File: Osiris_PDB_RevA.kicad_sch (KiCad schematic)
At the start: 22 parts, among them J1 XT60, Q1 ISC015N06NM5LF2, Q2 ISC015N06NM5LF2, U1 LTC4368IMS-1-PBF, U2 INA228AIDGSR, U3 TPS7A1633DGNR

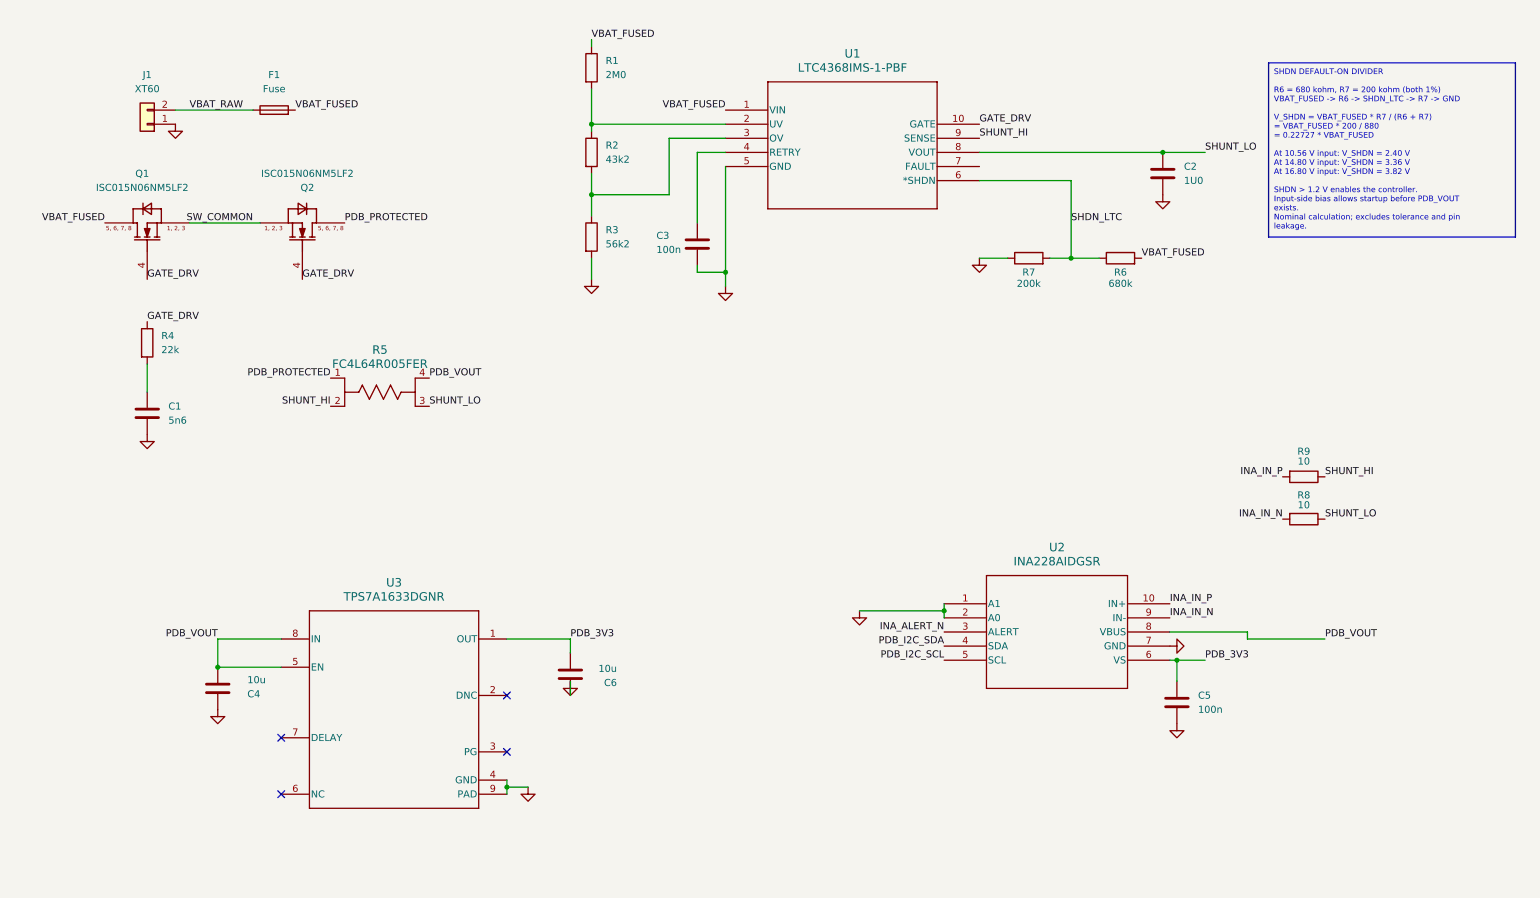
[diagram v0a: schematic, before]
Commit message: Consolidate Rev A schematic, component libraries and readiness review
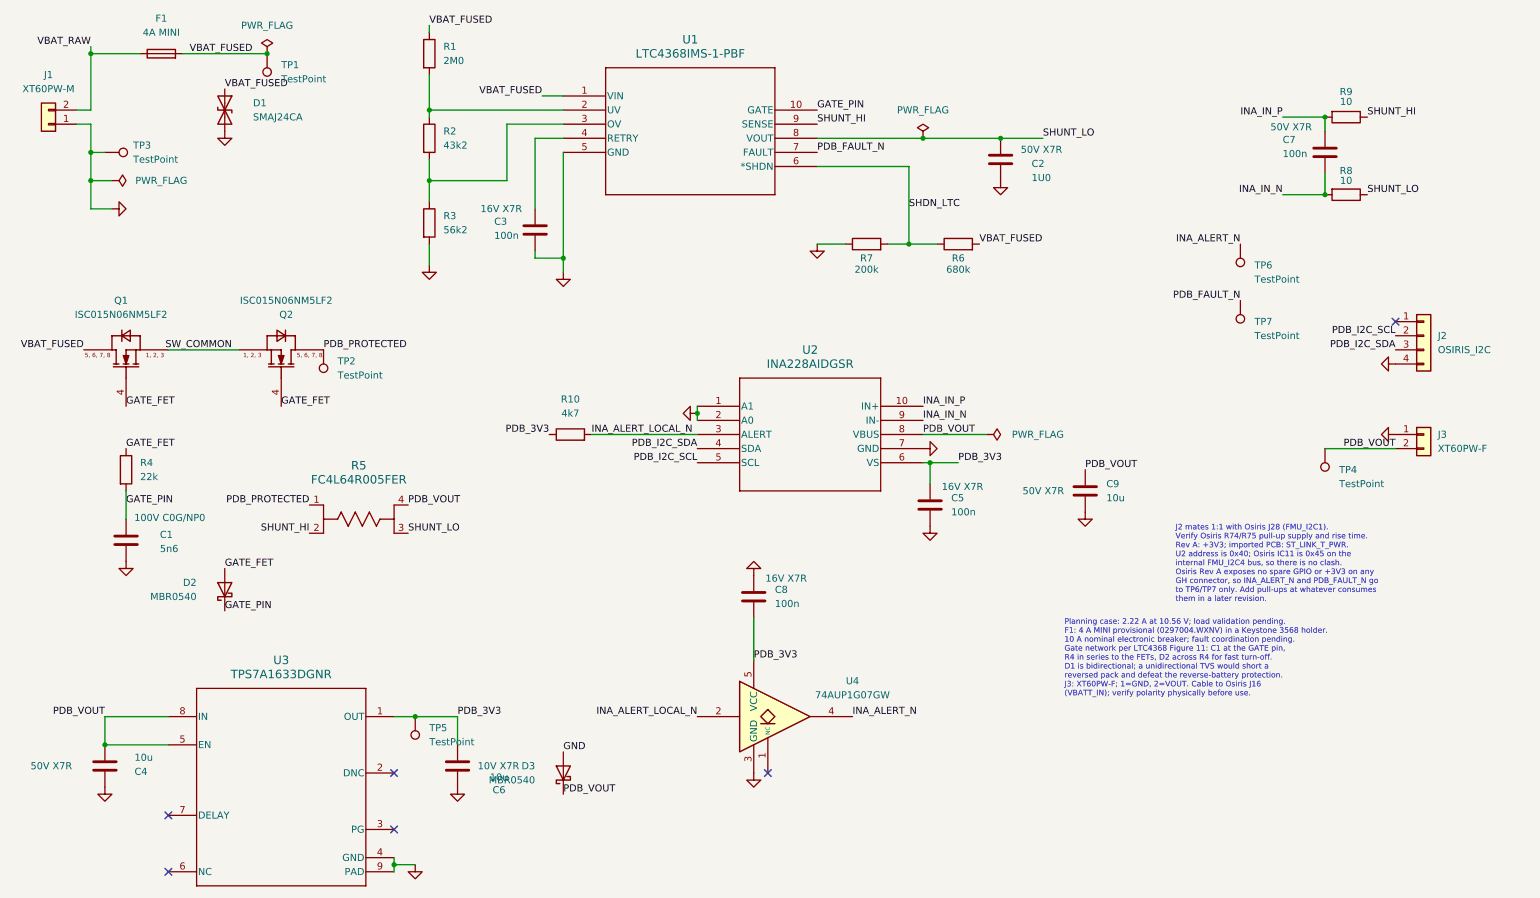
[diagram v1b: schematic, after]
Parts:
- added C7, C8: 100n, Capacitor_SMD:C_0603_1608Metric, symbol Device:C
- added C9: 10u, Capacitor_SMD:C_1206_3216Metric, symbol Device:C
- added D1: SMAJ24CA, Diode_SMD:D_SMA, symbol Device:D_TVS
- added D2, D3: MBR0540, Diode_SMD:D_SOD-123, symbol Device:D_Schottky
- added J2: OSIRIS_I2C, Connector_JST:JST_GH_BM04B-GHS-TBT_1x04-1MP_P1.25mm_Vertical, symbol Connector_Generic:Conn_01x04
- added J3: XT60PW-F, Connector_AMASS:AMASS_XT60PW-F_1x02_P7.20mm_Horizontal, symbol PDB_Symbols:XT60PW_F
- added R10: 4k7, Resistor_SMD:R_0805_2012Metric, symbol Device:R
- added TP1, TP2, TP3, TP4, TP5, TP6, TP7: TestPoint, TestPoint:TestPoint_Pad_D1.5mm, symbol Connector:TestPoint
- added U4: 74AUP1G07GW, Package_TO_SOT_SMD:SOT-353_SC-70-5, symbol 74xGxx:74AUP1G07
- C1: footprint (none) -> Capacitor_SMD:C_0805_2012Metric; MPN (none) -> C2012C0G2A562J125AA; Manufacturer (none) -> TDK; Selection_Status (none) -> CGATE at the U1 GATE pin per requirements D2; sets the 6.25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
- C2: footprint (none) -> Capacitor_SMD:C_0805_2012Metric; MPN (none) -> C2012X7R1H105K125AB; Manufacturer (none) -> TDK; Selection_Status (none) -> Nominal specification verified; DC-bias and circuit validat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
- C3, C5: footprint (none) -> Capacitor_SMD:C_0603_1608Metric; MPN (none) -> C0603C104K4RACTU; Manufacturer (none) -> KEMET; Selection_Status (none) -> Nominal specification verified; DC-bias and circuit validat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
- C4: footprint (none) -> Capacitor_SMD:C_1206_3216Metric; MPN (none) -> C3216X7R1H106K160AC; Manufacturer (none) -> TDK; Selection_Status (none) -> 10 uF local U3 input capacitor on protected PDB_VOUT.
- C6: footprint (none) -> Capacitor_SMD:C_0805_2012Metric; MPN (none) -> C2012X7R1A106K125AC; Manufacturer (none) -> TDK; Selection_Status (none) -> Nominal specification verified; DC-bias and circuit validat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
- F1: value Fuse -> 4A MINI; footprint (none) -> Fuse:Fuseholder_Blade_Mini_Keystone_3568; Holder_Datasheet (none) -> ${KIPRJMOD}/Datasheets/Keystone_3568.pdf; Holder_MPN (none) -> 3568; Holder_Manufacturer (none) -> Keystone Electronics; MPN (none) -> 0297004.WXNV; Manufacturer (none) -> Littelfuse; Selection_Status (none) -> PROVISIONAL 4 A candidate. 2.22 A is an assumed operating s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
- J1: value XT60 -> XT60PW-M; footprint (none) -> Connector_AMASS:AMASS_XT60PW-M_1x02_P7.20mm_Horizontal; MPN (none) -> XT60PW-M; Manufacturer (none) -> AMASS; Selection_Status (none) -> Assigned; verify cable mating, polarity and board-edge clea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
- Q1, Q2: footprint (none) -> PDB_Footprints:ISC015N06NM5LF2_TDSON8FL; MPN (none) -> ISC015N06NM5LF2; Manufacturer (none) -> Infineon
- R1, R2: footprint (none) -> Resistor_SMD:R_0805_2012Metric; Selection_Status (none) -> Package assigned; MPN and power/tolerance validation pending; Tolerance (none) -> 1%
- R3, R6, R7, R8, R9: footprint (none) -> Resistor_SMD:R_0805_2012Metric; Selection_Status (none) -> Package assigned; MPN and power/tolerance validation pending
- R4: footprint (none) -> Resistor_SMD:R_0805_2012Metric; Selection_Status (none) -> RGATE in the LTC4368 Figure 11 series position per requirem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; Tolerance (none) -> 1%
- R5: MPN (none) -> FC4L64R005FER; Manufacturer (none) -> Ohmite
- U1: footprint MS_10_ADI -> PDB_Footprints:MS_10-MSOP_ADI; MPN (none) -> LTC4368IMS-1#PBF; Manufacturer (none) -> Analog Devices
- U2: footprint VSSOP10_DGS_TEX -> PDB_Footprints:VSSOP10_DGS_TEX; MPN (none) -> INA228AIDGSR; Manufacturer (none) -> Texas Instruments
- U3: footprint DGN0008C_N -> PDB_Footprints:DGN0008C_N; MPN (none) -> TPS7A1633DGNR; Manufacturer (none) -> Texas Instruments; Selection_Status (none) -> Supplied from protected PDB_VOUT; loses power during a trip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
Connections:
- net GND: now also C8.1, C9.2, D1.2 (A2), D3.2 (A), J2.4 (Pin_4), J3.1 (-), TP3.1, U4.3 (GND)
- net INA_ALERT_N: now also TP6.1, U4.4; no longer U2.3 (ALERT)
- net INA_IN_N: now also C7.2
- net INA_IN_P: now also C7.1
- net PDB_3V3: now also C8.2, R10.1, TP5.1, U4.5 (VCC)
- net PDB_I2C_SCL: now also J2.2 (Pin_2)
- net PDB_I2C_SDA: now also J2.3 (Pin_3)
- net PDB_PROTECTED: now also TP2.1
- net PDB_VOUT: now also C9.1, D3.1 (K), J3.2 (+), TP4.1
- net VBAT_FUSED: now also D1.1 (A1), TP1.1
- net GATE_PIN: now reaches C1.1, R4.2
- net GATE_PIN: now also U1.10 (GATE), D2.1 (K)
- net PDB_FAULT_N: now reaches U1.7 (FAULT)
- net PDB_FAULT_N: now also TP7.1
- net GATE_DRV renamed GATE_FET
- net GATE_FET: now also D2.2 (A); no longer U1.10 (GATE)
- new net INA_ALERT_LOCAL_N: R10.2, U2.3 (ALERT), U4.2
- no-connect marks 4 -> 6
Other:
- note added: "J2 mates 1:1 with Osiris J28 (FMU_I2C1). Verify Osiris R74/R75 pull-up supply and rise time. Rev A: +3V3; imported PCB: ST_LINK_T_PWR. U2 address is 0x40; Osiris IC11 is 0x45 on the internal FMU_I2C4 bus, so there is no clash. Osiris Rev A exposes no spare GPIO or +3V3 on any GH connector, so INA_ALERT_N and PDB_FAULT_N go to TP6/TP7 only. Add pull-ups at whatever consumes them in a later revisio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"
- note added: "Planning case: 2.22 A at 10.56 V; load validation pending. F1: 4 A MINI provisional (0297004.WXNV) in a Keystone 3568 holder. 10 A nominal electronic breaker; fault coordination pending. Gate network per LTC4368 Figure 11: C1 at the GATE pin, R4 in series to the FETs, D2 across R4 for fast turn-off. D1 is bidirectional; a unidirectional TVS would short a reversed pack and defeat the reverse-batte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"
- moved on the sheet: C1, C2, C3, C4, C5, C6, F1, J1, Q1, Q2, R1, R2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
